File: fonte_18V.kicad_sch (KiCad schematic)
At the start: 12 parts, among them J101 IN, J102 Conn_01x02

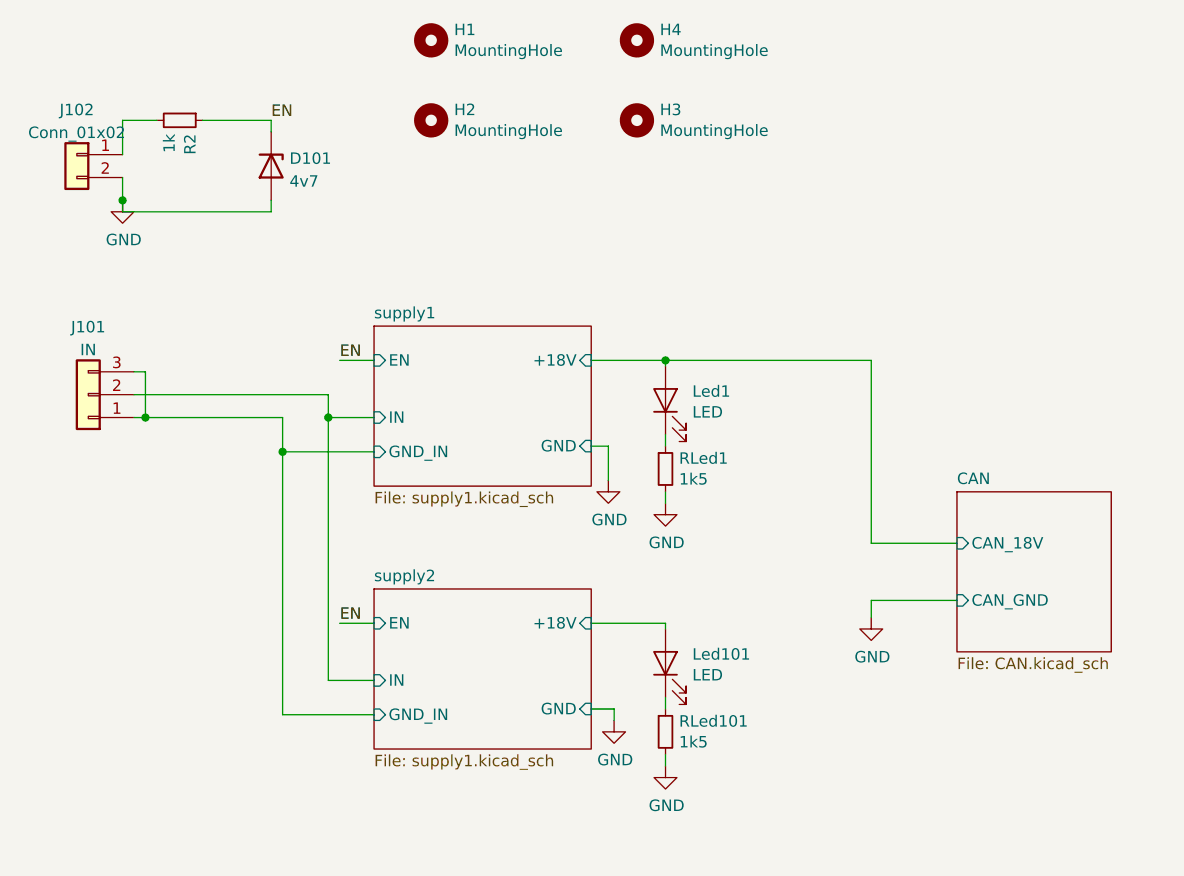
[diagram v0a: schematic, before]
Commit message: almost finished
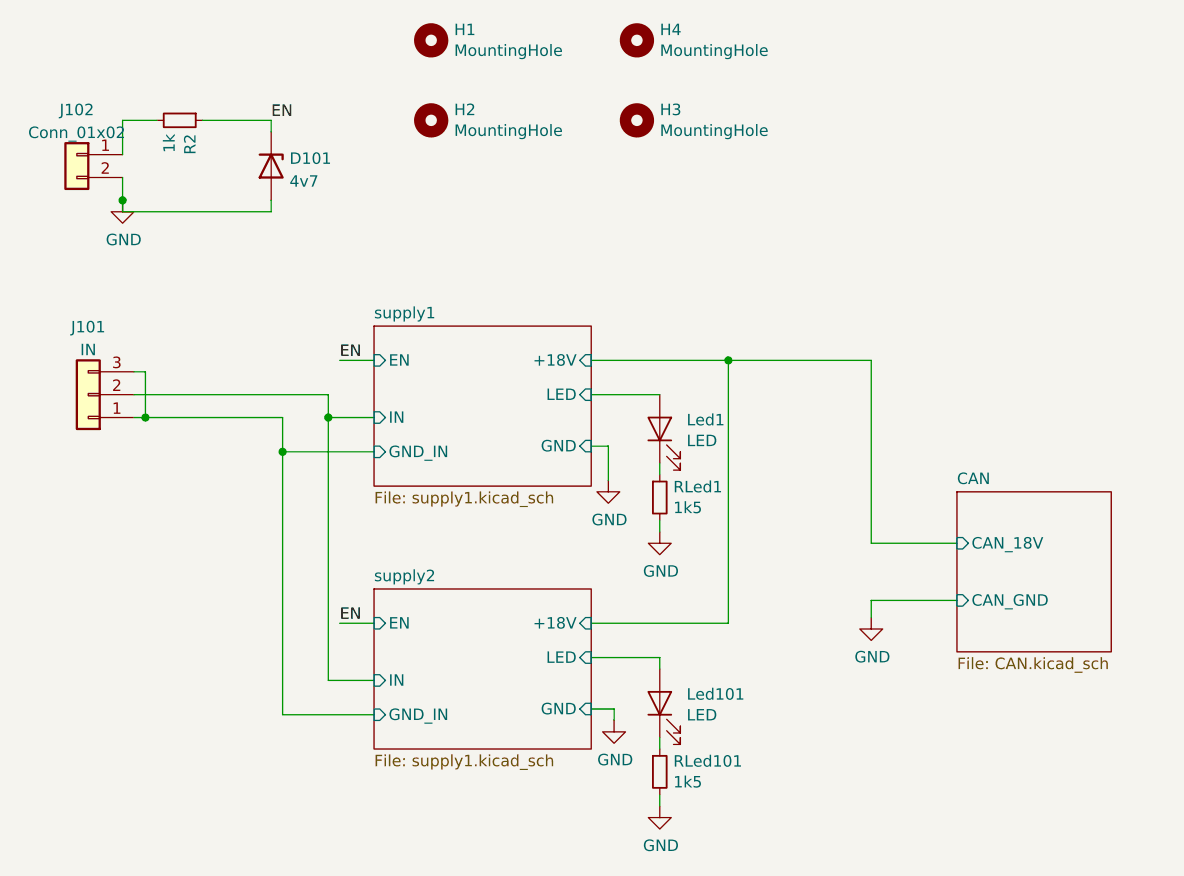
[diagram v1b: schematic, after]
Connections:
- net CAN/CAN_18V: no longer Led1.2 (A)
- net supply2/+18V renamed supply2/LED
- new net supply1/LED: Led1.2 (A)
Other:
- sheet supply1 ports: added LED; removed none
- sheet supply2 ports: added LED; removed none
- moved on the sheet: Led1, Led101, RLed1, RLed101
